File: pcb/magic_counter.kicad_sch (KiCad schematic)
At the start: 16 parts, among them J1 ISP-Port, J2 Serial Out, SW1 Random, U1 ATmega32A-P, Y1 Crystal

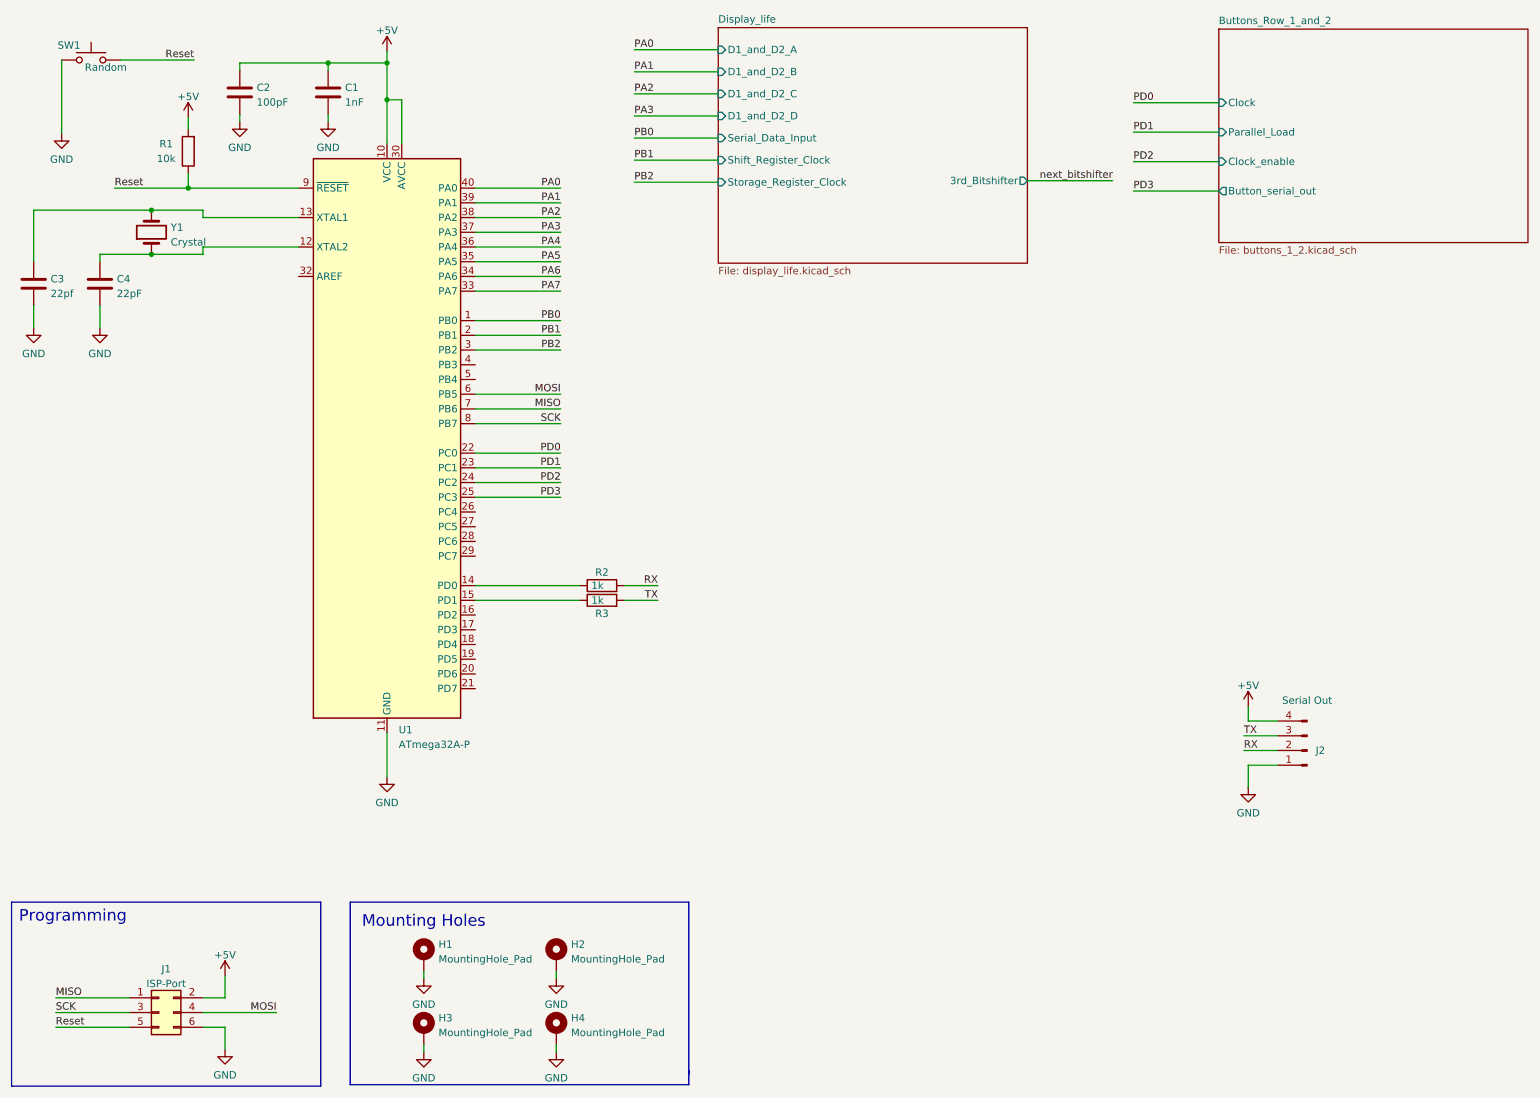
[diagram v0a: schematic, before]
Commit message: test 1
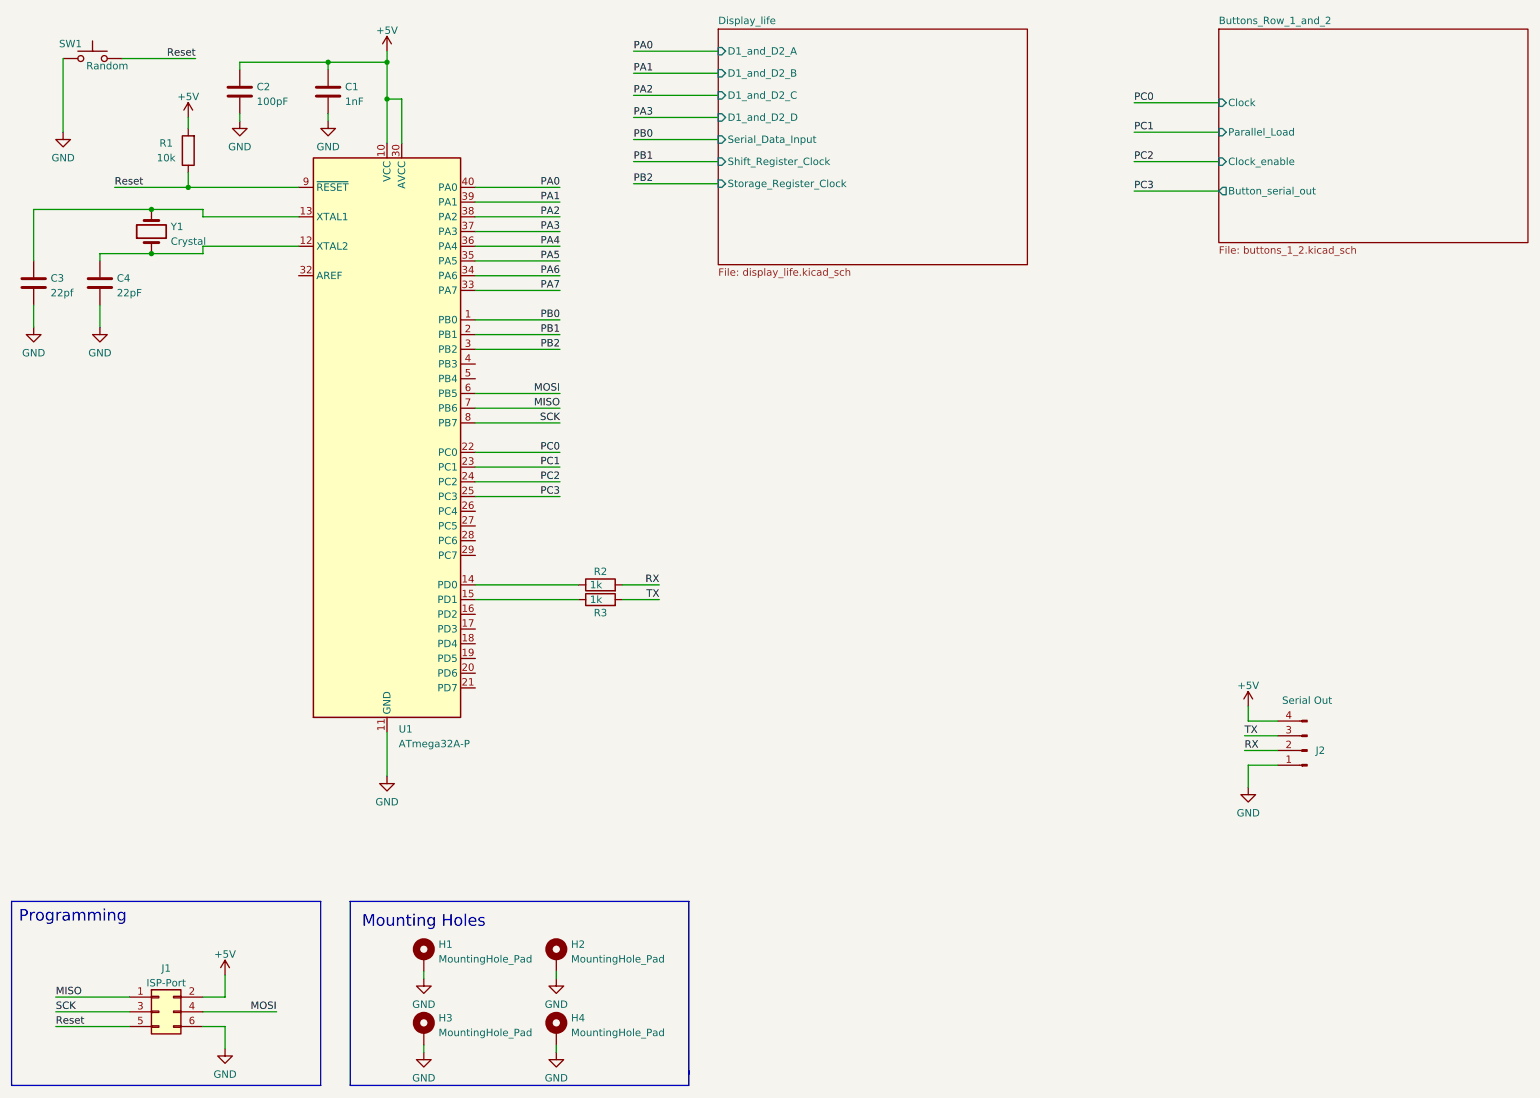
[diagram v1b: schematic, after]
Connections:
- net PD0 renamed PC0
- net PD1 renamed PC1
- net PD2 renamed PC2
- net PD3 renamed PC3
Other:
- sheet Display_life ports: added none; removed 3rd_Bitshifter
